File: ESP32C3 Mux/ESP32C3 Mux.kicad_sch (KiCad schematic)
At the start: 4 parts

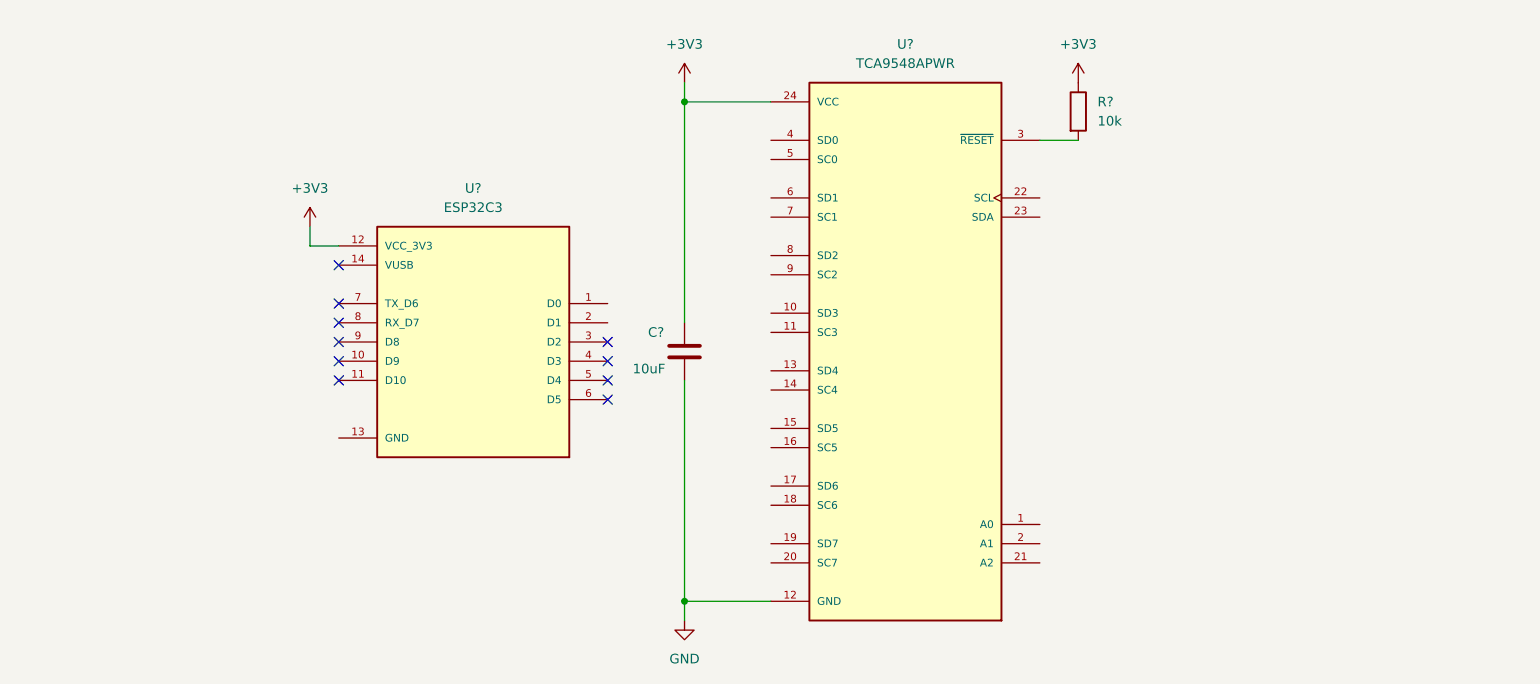
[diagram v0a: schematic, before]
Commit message: finished esp32 mux schematic
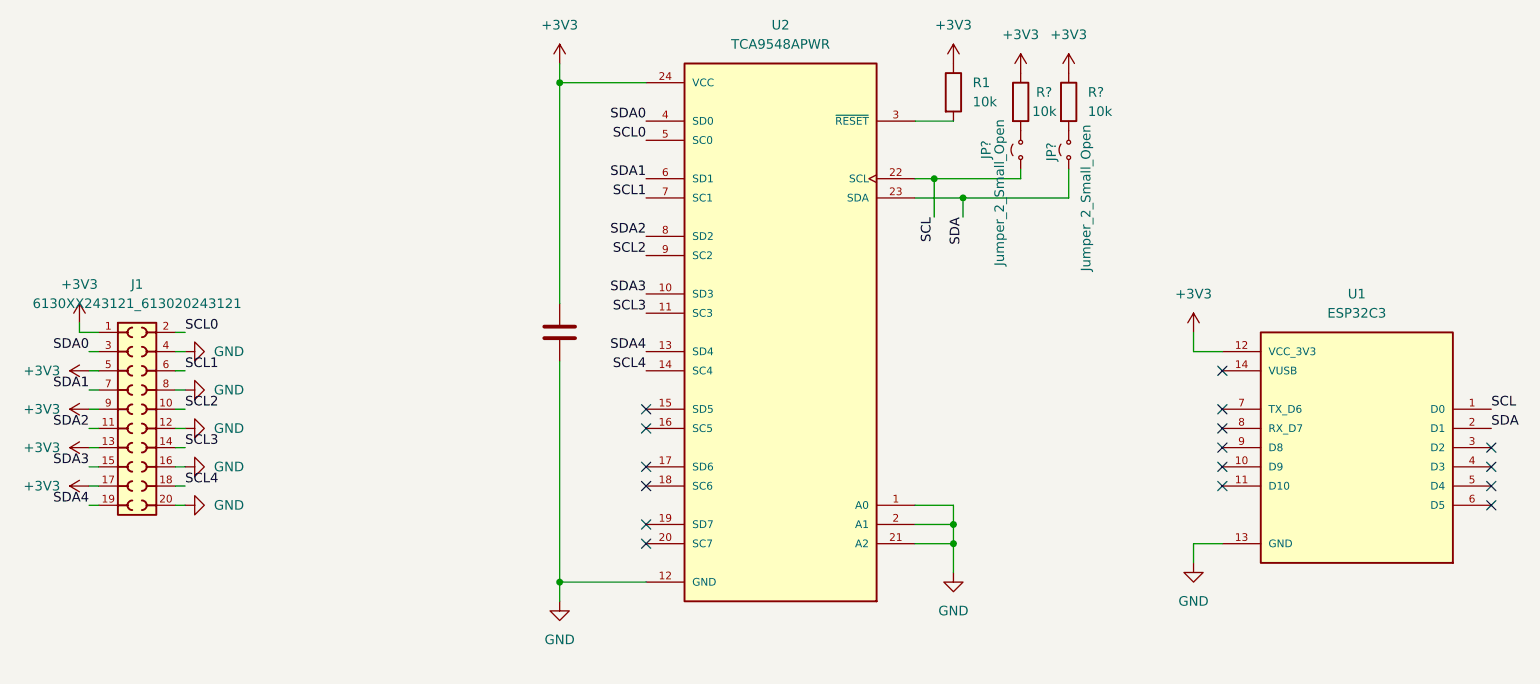
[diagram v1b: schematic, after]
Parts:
- added J1: 6130XX243121_613020243121, ESP32C3 Mux:613020243121, symbol ESP32C3Mux:6130XX243121_613020243121
- added JP? (x2): Jumper_2_Small_Open, symbol Jumper:Jumper_2_Small_Open
- added R? (x2): 10k, symbol Device:R
- gave numbers to parts that had none: 4
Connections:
- net +3V3: now also J1.1, J1.13, J1.17, J1.5, J1.9, R?.1, R?.1
- net GND: now also U1.13 (GND), U2.1 (A0), U2.2 (A1), U2.21 (A2), J1.12, J1.16, J1.20, J1.4, J1.8
- net SDA3: now reaches U2.10 (SD3)
- net SDA3: now also J1.15
- net SCL3: now reaches U2.11 (SC3)
- net SCL3: now also J1.14
- net SDA4: now reaches U2.13 (SD4)
- net SDA4: now also J1.19
- net SCL4: now reaches U2.14 (SC4)
- net SCL4: now also J1.18
- net SCL: now reaches U2.22 (SCL)
- net SCL: now also U1.1 (D0), JP?.1 (A)
- net SDA: now reaches U2.23 (SDA)
- net SDA: now also U1.2 (D1), JP?.1 (A)
- net SDA0: now reaches U2.4 (SD0)
- net SDA0: now also J1.3
- net SCL0: now reaches U2.5 (SC0)
- net SCL0: now also J1.2
- net SDA1: now reaches U2.6 (SD1)
- net SDA1: now also J1.7
- net SCL1: now reaches U2.7 (SC1)
- net SCL1: now also J1.6
- net SDA2: now reaches U2.8 (SD2)
- net SDA2: now also J1.11
- net SCL2: now reaches U2.9 (SC2)
- net SCL2: now also J1.10
- new net: JP?.2 (B), R?.2 (x2)
- no-connect marks 10 -> 16
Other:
- moved on the sheet: R1, U1, U2
